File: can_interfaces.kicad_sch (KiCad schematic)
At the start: 38 parts, among them SW1 SW_DIP_x03, U13 MCP2562FD, U14 MCP2562FD, U15 MCP2562FD

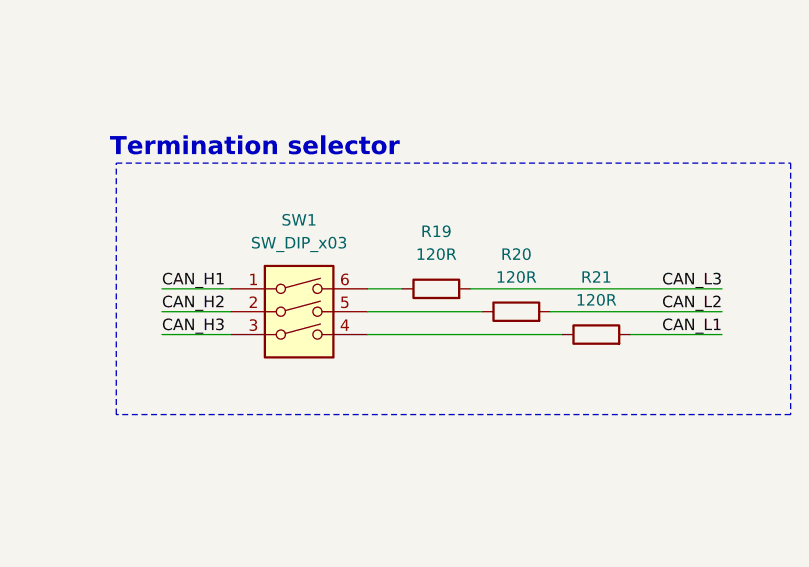
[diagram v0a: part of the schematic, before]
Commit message: feat: started writing BOM
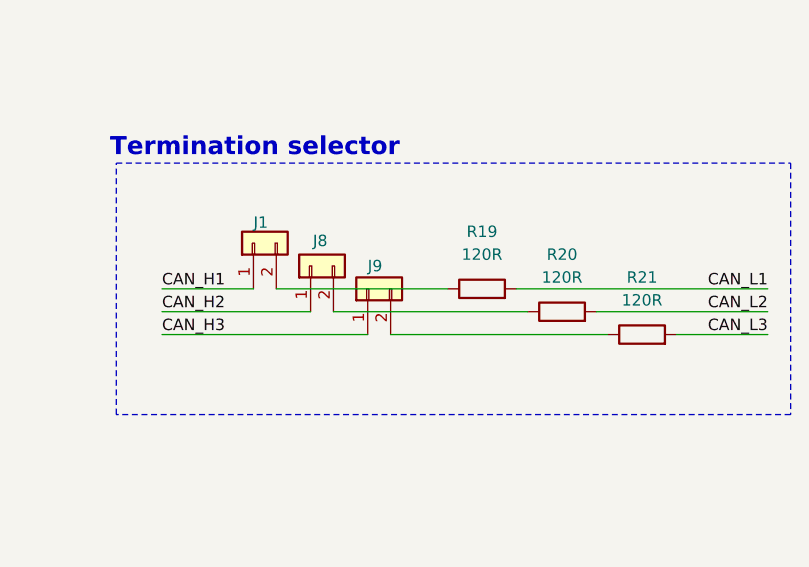
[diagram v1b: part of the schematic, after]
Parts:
- removed SW1: SW_DIP_x03, Button_Switch_SMD:SW_DIP_SPSTx03_Slide_6.7x9.18mm_W6.73mm_P2.54mm_LowProfile_JPin, symbol Switch:SW_DIP_x03
- added J1, J8, J9: Conn_01x02, Connector_PinHeader_2.00mm:PinHeader_1x02_P2.00mm_Vertical, symbol Connector_Generic:Conn_01x02
- C33, C34, C35, C36, C37, C38, C39, C40, C41, C42, C43, C44: LCSC Part # (none) -> C1644; MOUSER PN (none) -> 581-06031U150FAT2A
- C45, C46, C47, C48, C49, C50: LCSC Part # (none) -> C14663; MOUSER PN (none) -> 963-MAJCU168BB7104KT
- D19, D20, D21: LCSC Part # (none) -> C284104; MOUSER PN (none) -> 637-NUP2105L
- D22: now left out of the parts list
- FL1, FL2, FL3: LCSC Part # (none) -> C88056; MOUSER PN (none) -> 810-ACT45B1012PTL003
- R19, R20, R21: LCSC Part # (none) -> C22787; MOUSER PN (none) -> 652-CR0603-JW-121ELF
- R44, R45, R46, R47, R48, R49: LCSC Part # (none) -> C23140; MOUSER PN (none) -> 603-AF0603JR-0733RL
- U13, U14, U15: LCSC Part # (none) -> C511335; MOUSER PN (none) -> 579-MCP2562FD-H/SN
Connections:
- net CAN_H1: now also J1.1 (Pin_1)
- net CAN_H2: now also J8.1 (Pin_1)
- net CAN_H3: now also J9.1 (Pin_1)
- net CAN_L1: now also R19.2; no longer R21.2
- net CAN_L3: now also R21.2; no longer R19.2
- net at R21.1: now also J9.2 (Pin_2)
- net at R20.1: now also J8.2 (Pin_2)
- net at R19.1: now also J1.2 (Pin_2)
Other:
- moved on the sheet: R19, R20, R21
